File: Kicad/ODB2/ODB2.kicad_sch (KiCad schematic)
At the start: 31 parts, among them U1 STM32F412ZGTx

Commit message: ajout footprints
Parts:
- RST_C1: footprint (none) -> Capacitor_SMD:C_0805_2012Metric
- RST_R1: footprint (none) -> Resistor_SMD:R_0805_2012Metric
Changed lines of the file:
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@@
 			)
 		)
-		(property "Footprint" ""
+		(property "Footprint" "Resistor_SMD:R_0805_2012Metric"
 			(at 144.272 49.53 90)
 			(effects
@@
 			)
 		)
-		(property "Footprint" ""
+		(property "Footprint" "Capacitor_SMD:C_0805_2012Metric"
 			(at 147.0152 64.77 0)
 			(effects

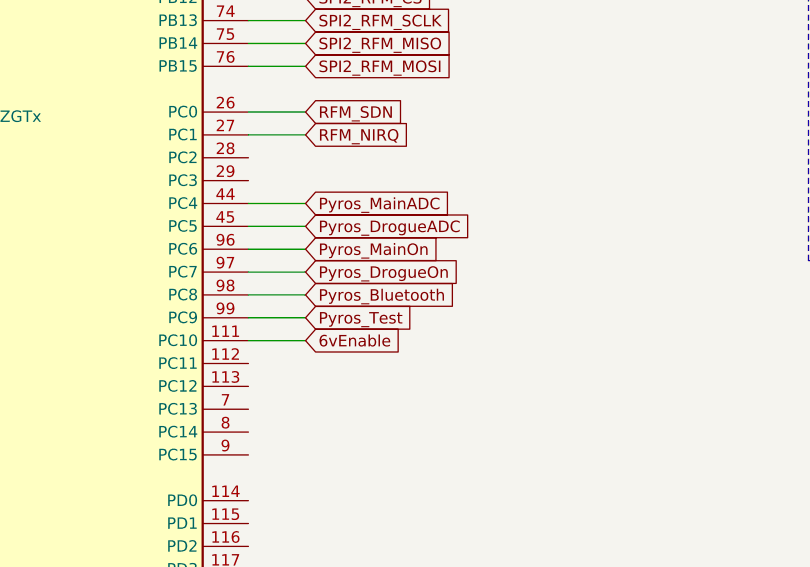
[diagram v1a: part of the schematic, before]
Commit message: revision logic
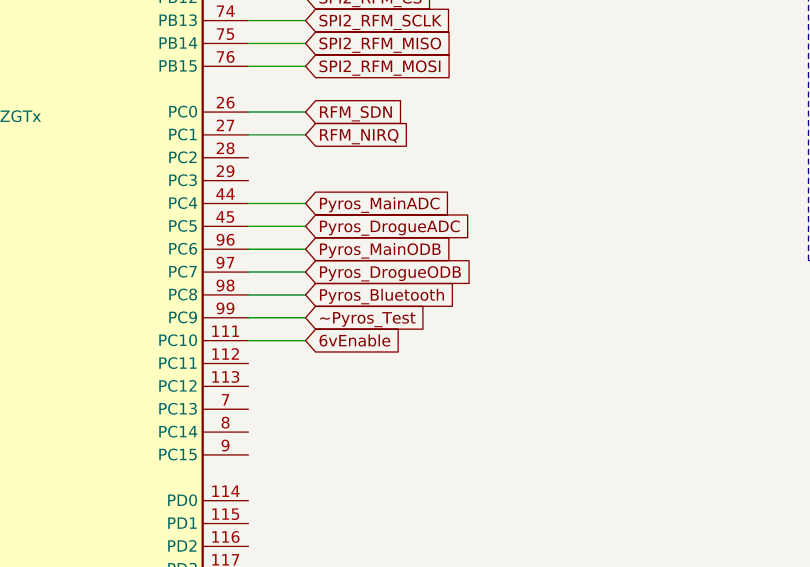
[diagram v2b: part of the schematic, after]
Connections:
- net Pyros_DrogueOn renamed Pyros_DrogueODB
- net Pyros_MainOn renamed Pyros_MainODB
- net Pyros_Test renamed ~Pyros_Test
